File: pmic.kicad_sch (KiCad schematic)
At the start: 1 part, among them U2 RK809-1

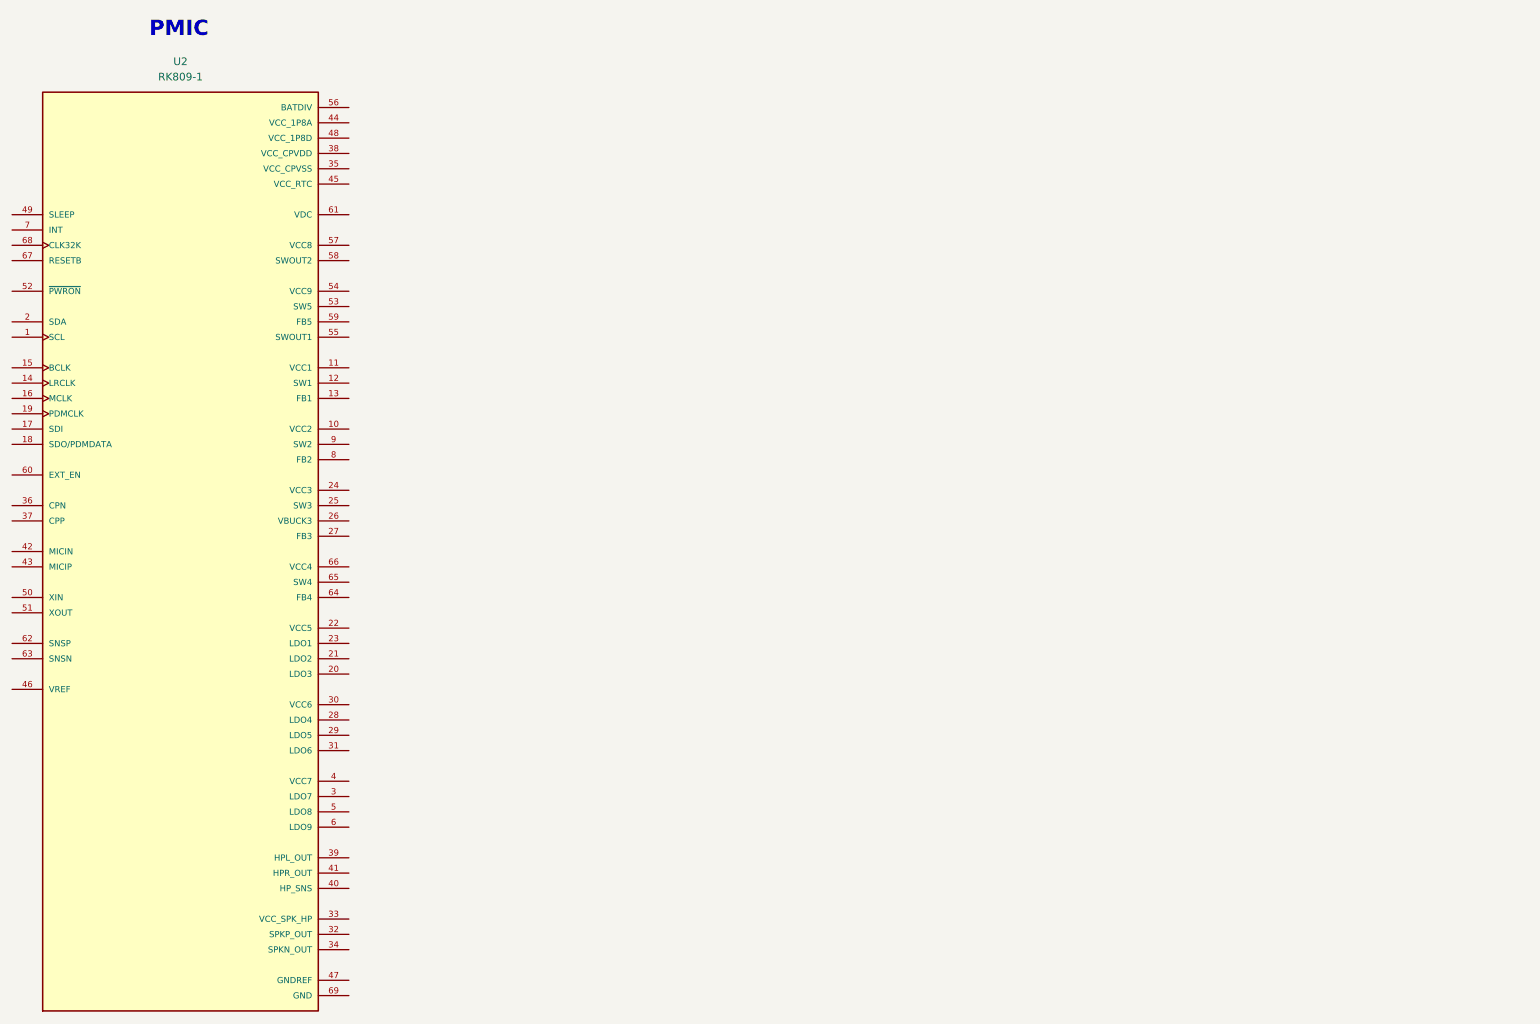
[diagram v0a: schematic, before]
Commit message: pmic
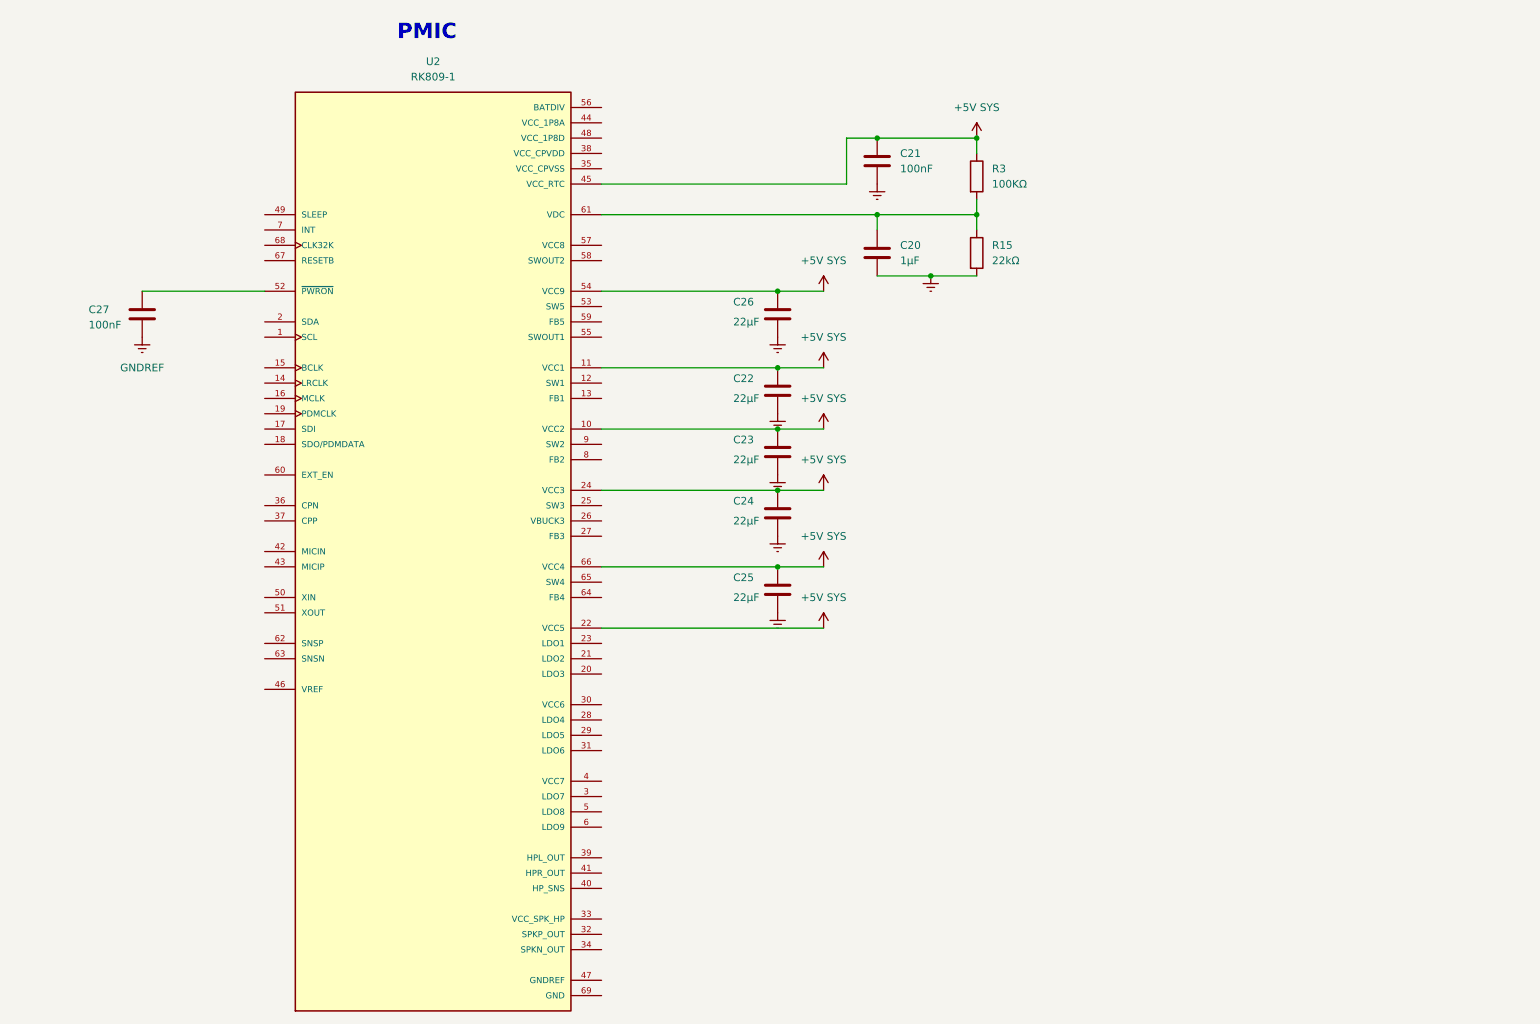
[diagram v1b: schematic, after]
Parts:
- added C20: 1µF, symbol Device:C
- added C21, C27: 100nF, symbol Device:C
- added C22, C23, C24, C25, C26: 22µF, symbol Device:C
- added R15: 22kΩ, symbol Device:R
- added R3: 100KΩ, symbol Device:R
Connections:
- net +5V SYS: now reaches U2.10 (VCC2)
- net +5V SYS: now also U2.11 (VCC1), U2.22 (VCC5), U2.24 (VCC3), U2.45 (VCC_RTC), U2.54 (VCC9), U2.66 (VCC4), C21.1, C22.1, C23.1, C24.1, C25.1, C26.1, R3.1
- net at U2.52 (~{PWRON}): now also C27.1
- net at U2.61 (VDC): now also C20.1, R15.1, R3.2
- new net GNDREF: C20.2, C21.2, C22.2, C23.2, C24.2, C25.2, C26.2, C27.2, R15.2
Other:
- moved on the sheet: U2

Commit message: pmic
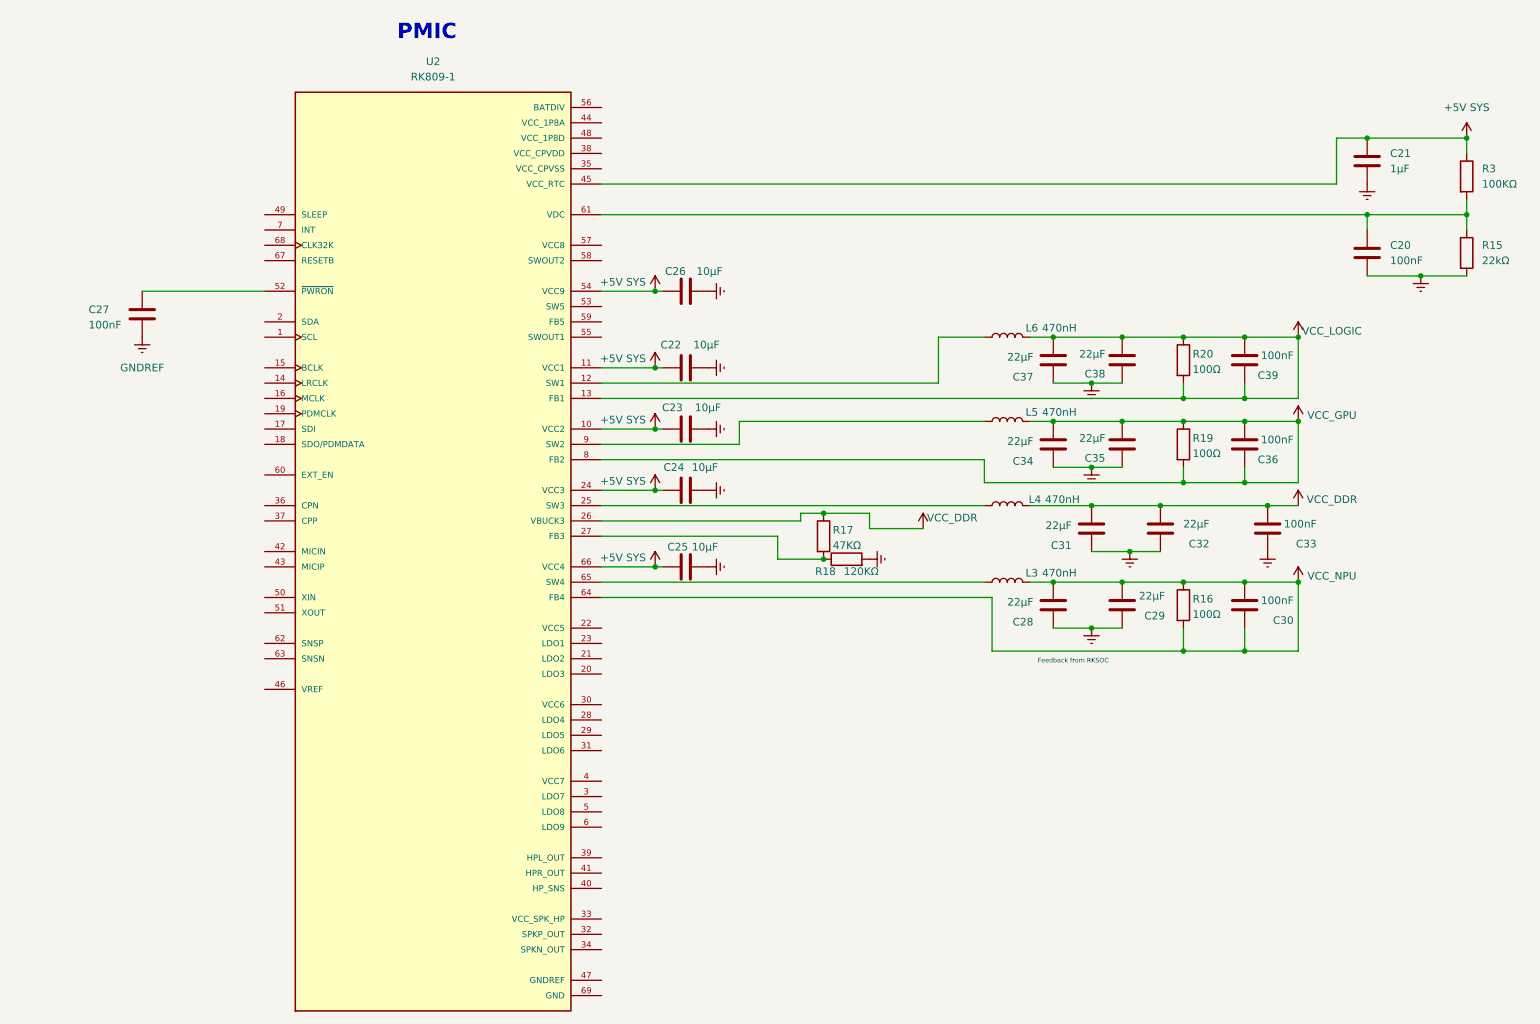
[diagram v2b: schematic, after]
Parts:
- added C28, C29, C31, C32, C34, C35, C37, C38: 22µF, symbol Device:C
- added C30, C33, C36, C39: 100nF, symbol Device:C
- added L3, L4, L5, L6: 470nH, symbol Device:L
- added R16, R19, R20: 100Ω, symbol Device:R
- added R17: 47KΩ, symbol Device:R
- added R18: 120KΩ, symbol Device:R
- C20: value 1µF -> 100nF
- C21: value 100nF -> 1µF
- C22, C23, C24, C25, C26: value 22µF -> 10µF
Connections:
- net +5V SYS: now also C25.2; no longer C25.1, U2.22 (VCC5)
- net GNDREF: now also C25.1, C28.2, C29.2, C31.2, C32.2, C33.2, C34.2, C35.2, C37.2, C38.2, R18.2; no longer C25.2
- net at U2.12 (SW1): now also L6.1
- net VCC_LOGIC: now reaches U2.13 (FB1)
- net VCC_LOGIC: now also C37.1, C38.1, C39.1, C39.2, L6.2, R20.1, R20.2
- net at U2.25 (SW3): now also L4.1
- net VCC_DDR: now reaches U2.26 (VBUCK3)
- net VCC_DDR: now also C31.1, C32.1, C33.1, L4.2, R17.1
- net at U2.27 (FB3): now also R17.2, R18.1
- net VCC_NPU: now reaches U2.64 (FB4)
- net VCC_NPU: now also C28.1, C29.1, C30.1, C30.2, L3.2, R16.1, R16.2
- net at U2.65 (SW4): now also L3.1
- net VCC_GPU: now reaches U2.8 (FB2)
- net VCC_GPU: now also C34.1, C35.1, C36.1, C36.2, L5.2, R19.1, R19.2
- net at U2.9 (SW2): now also L5.1
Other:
- note added: "Feedback from RKSOC"
- moved on the sheet: C20, C21, C22, C23, C24, C25, C26, R15, R3
